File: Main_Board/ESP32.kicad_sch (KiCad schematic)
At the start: 26 parts, among them J1 RESET, J2 MAIN_UART, Q1 2N7002, U1 W25Q128JVS, U2 ESP32-S3-MINI-1U

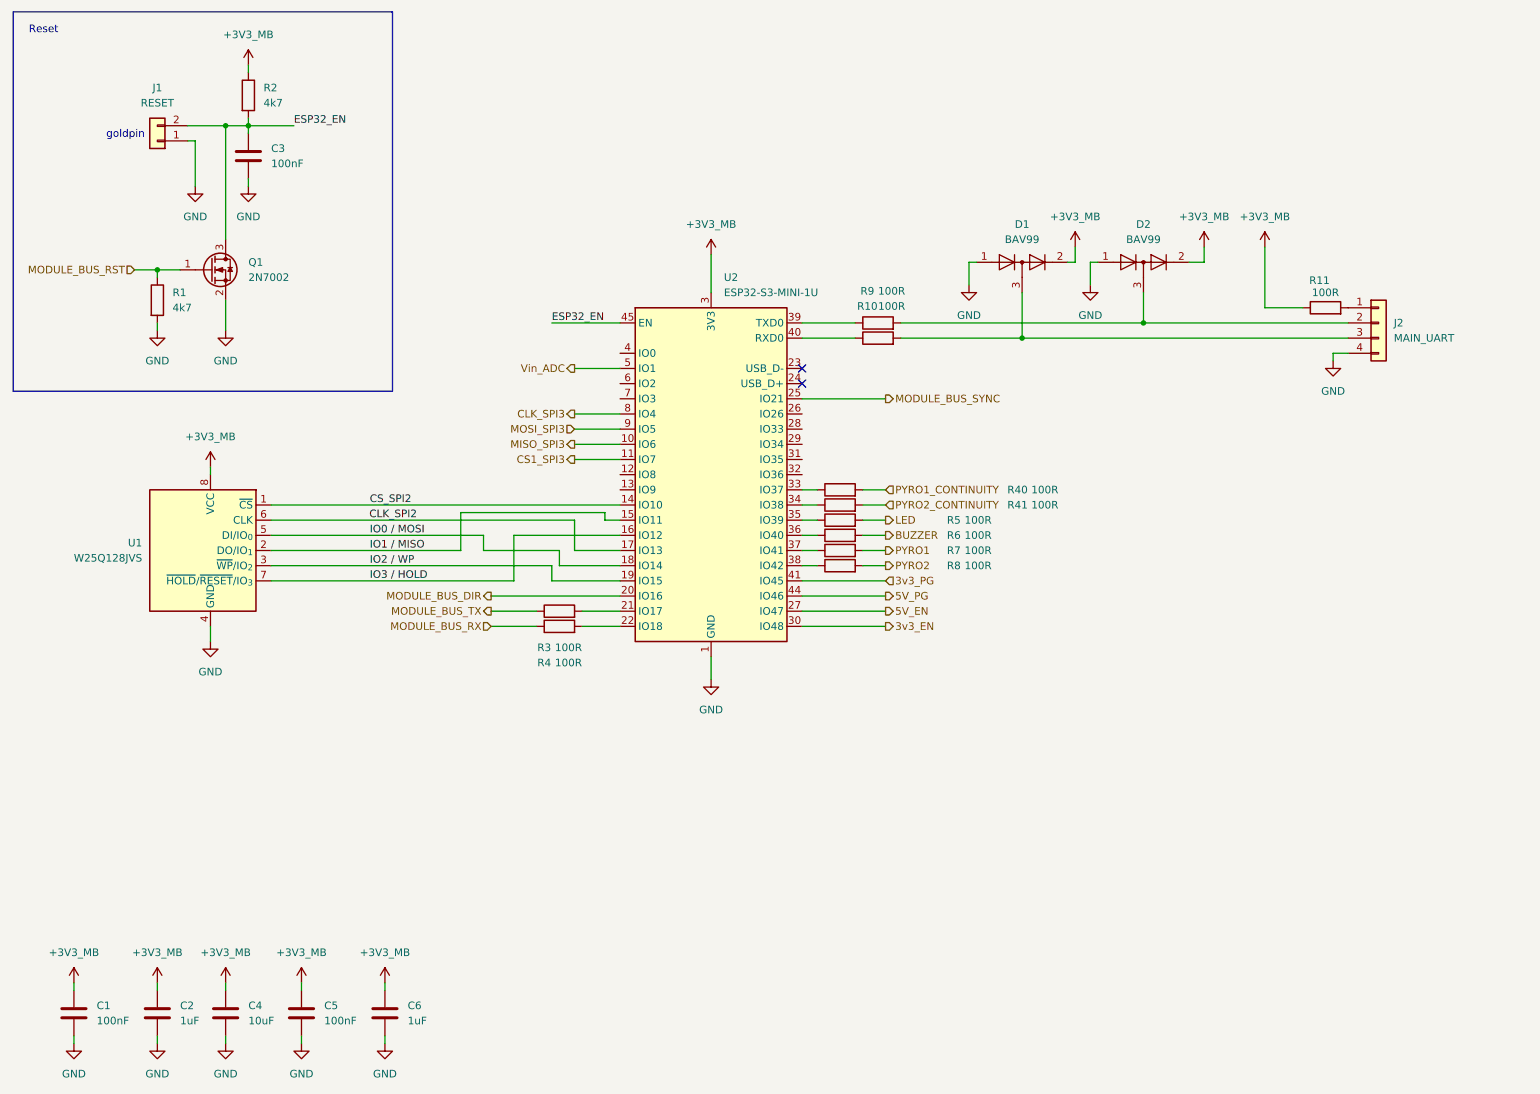
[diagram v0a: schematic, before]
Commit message: Fix schematic readibility
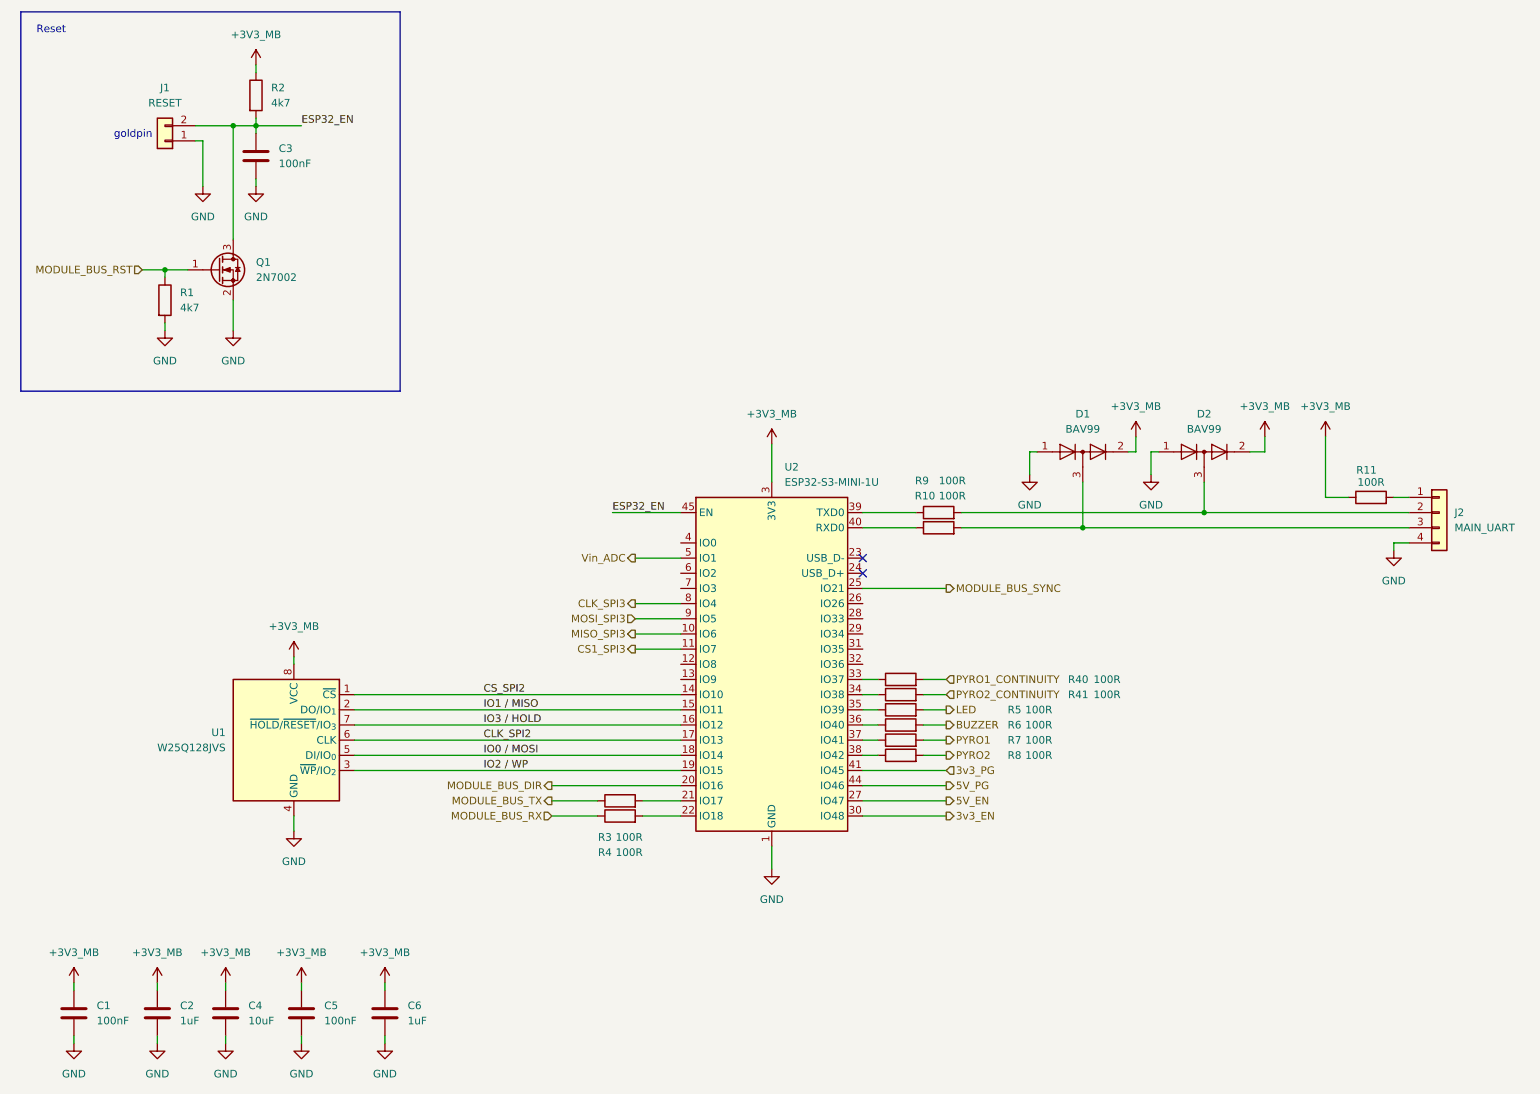
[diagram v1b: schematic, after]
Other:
- moved on the sheet: C3, D1, D2, J1, J2, Q1, R1, R10, R11, R2, R3, R4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
